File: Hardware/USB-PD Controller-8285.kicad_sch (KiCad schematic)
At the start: 27 parts, among them J1 Conn_01x07_Male, J10 Conn_Coaxial, J2 Conn_01x04_Male, J3 Conn_01x02_Male, J4 Conn_01x02_Male, J5 Conn_01x02_Male, J6 Conn_01x02_Male, J7 Conn_01x08_Male, J9 QWIIC_Stackable, Q1 UMH3N, U1 ESP8285H16, Y1 26.000MHz

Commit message: tweaks...
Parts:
- J7: LCSC (none) -> C2881786 + C2684732
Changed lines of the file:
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@@
+      (effects (font (size 1.27 1.27)) hide)
+    )
+    (property "LCSC" "C2881786 + C2684732" (id 4) (at 124.46 124.46 0)
       (effects (font (size 1.27 1.27)) hide)
     )

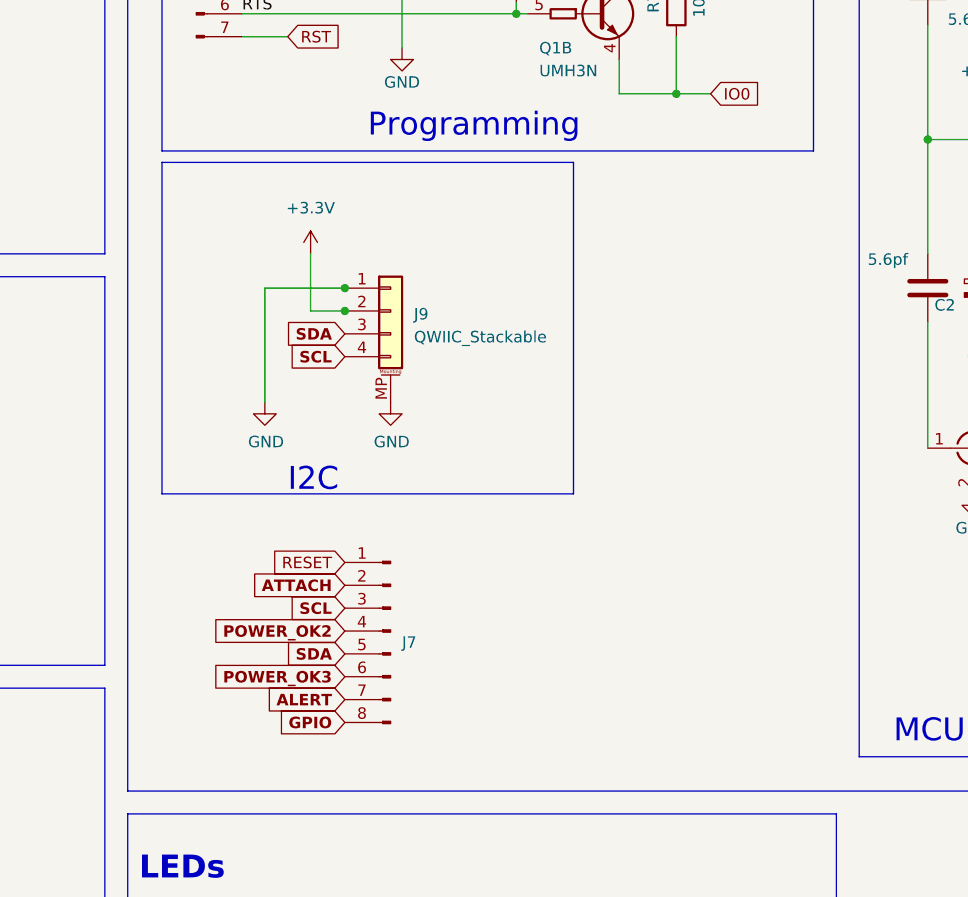
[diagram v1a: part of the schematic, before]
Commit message: messin' with the controller board
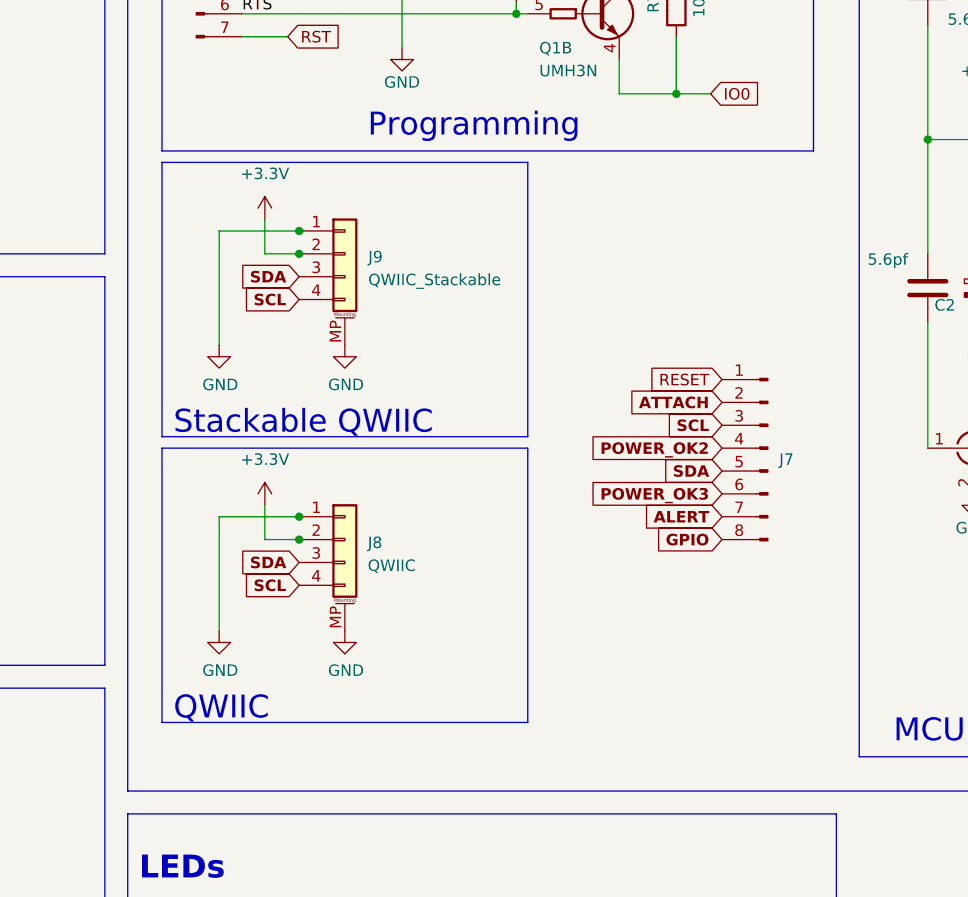
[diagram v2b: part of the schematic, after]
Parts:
- added J8: QWIIC, Connector_JST:JST_SH_BM04B-SRSS-TB_1x04-1MP_P1.00mm_Vertical, symbol Connector_QWIIC_Stackable:QWIIC_Stackable
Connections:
- net +3V3: now also J8.2 (Pin_2)
- net GND: now also J8.1 (Pin_1), J8.MP (MountPin)
- net SCL: now also J8.4 (Pin_4)
- net SDA: now also J8.3 (Pin_3)
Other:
- note added: "QWIIC"
- note added: "Stackable QWIIC"
- note removed: "I2C"
- moved on the sheet: J7, J9
